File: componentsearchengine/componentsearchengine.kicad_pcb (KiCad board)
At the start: 2 copper layers, 28 x 19 mm, 1 part, among them X1 X1G0044810050_SG7050CAN_2.048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

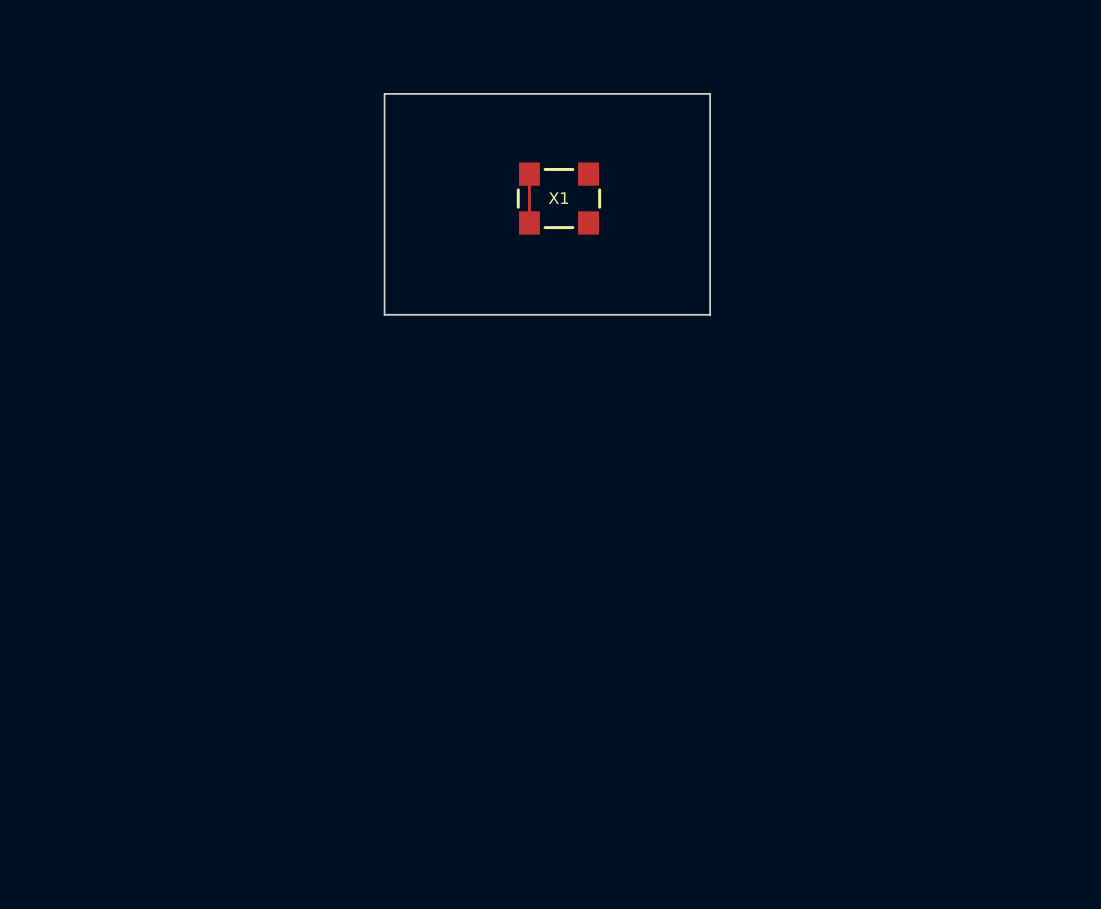
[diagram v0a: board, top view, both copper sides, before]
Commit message: Goodnight.
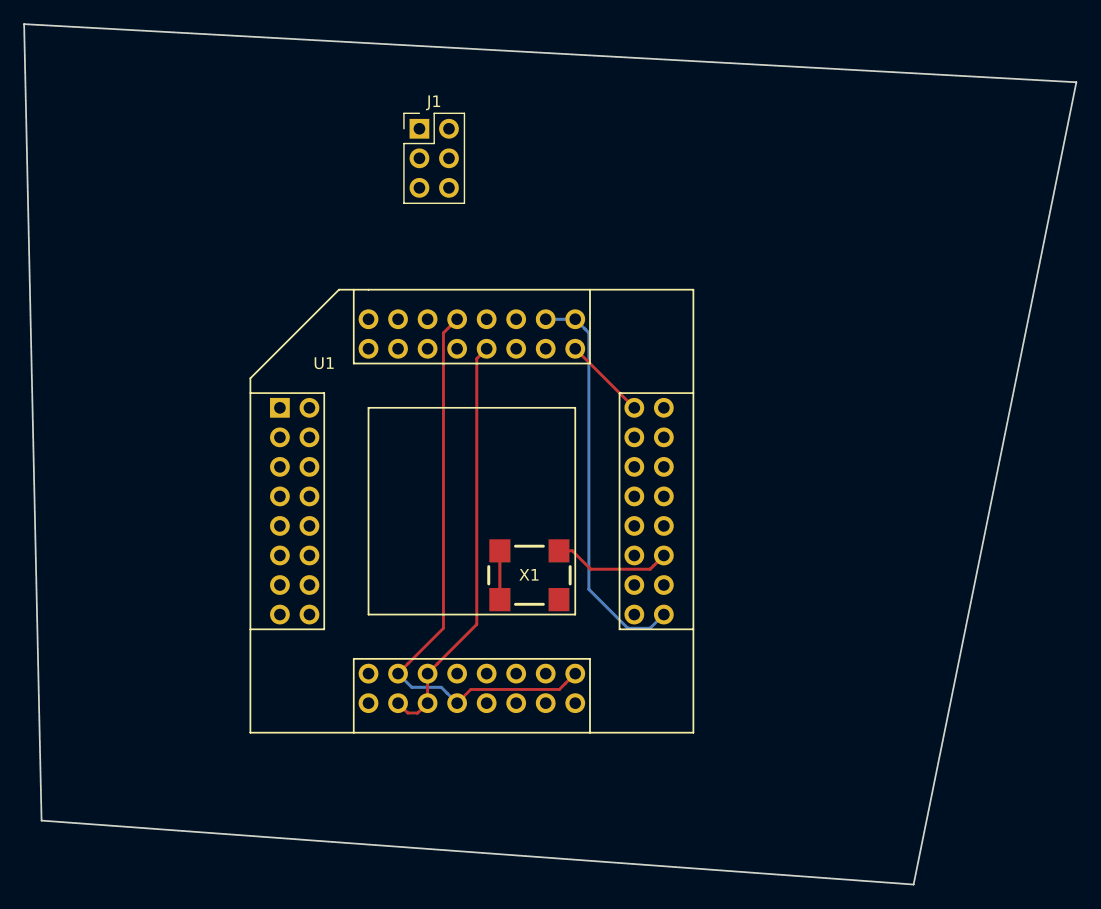
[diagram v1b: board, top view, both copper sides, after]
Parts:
- added J1: Conn_02x03_Counter_Clockwise, Pin_Headers:Pin_Header_Straight_2x03_Pitch2.54mm, F.Cu at (84.0, 32.0)
- added U1: ADS1299-4PAG, prj_lib_fp:xQFP_64_to_2.54mm_adapter, F.Cu at (72.0, 56.0)
- moved X1 32.5 mm to (93.5, 70.4)
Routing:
- net Net-(U1-Pad20): track 0.00 -> 49.9 mm
- net Net-(U1-Pad19): track 0.00 -> 35.8 mm
- net Net-(U1-Pad33): track 0.00 -> 34.6 mm
- net Net-(U1-Pad37): track 0.00 -> 10.2 mm
- net Net-(U1-Pad48): track 0.00 -> 7.18 mm
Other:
- board size 28 x 19 mm -> 90.5 x 74 mm
